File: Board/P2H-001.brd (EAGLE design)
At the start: 94.9 x 72.4 mm, 29 parts, among them IC1 74LS157N, IC2 LTC485N, IC3 74LS07N, IC4 LTC485N, IC5 4066N, IC6 TLC5941NT, IC7 TLC5941NT

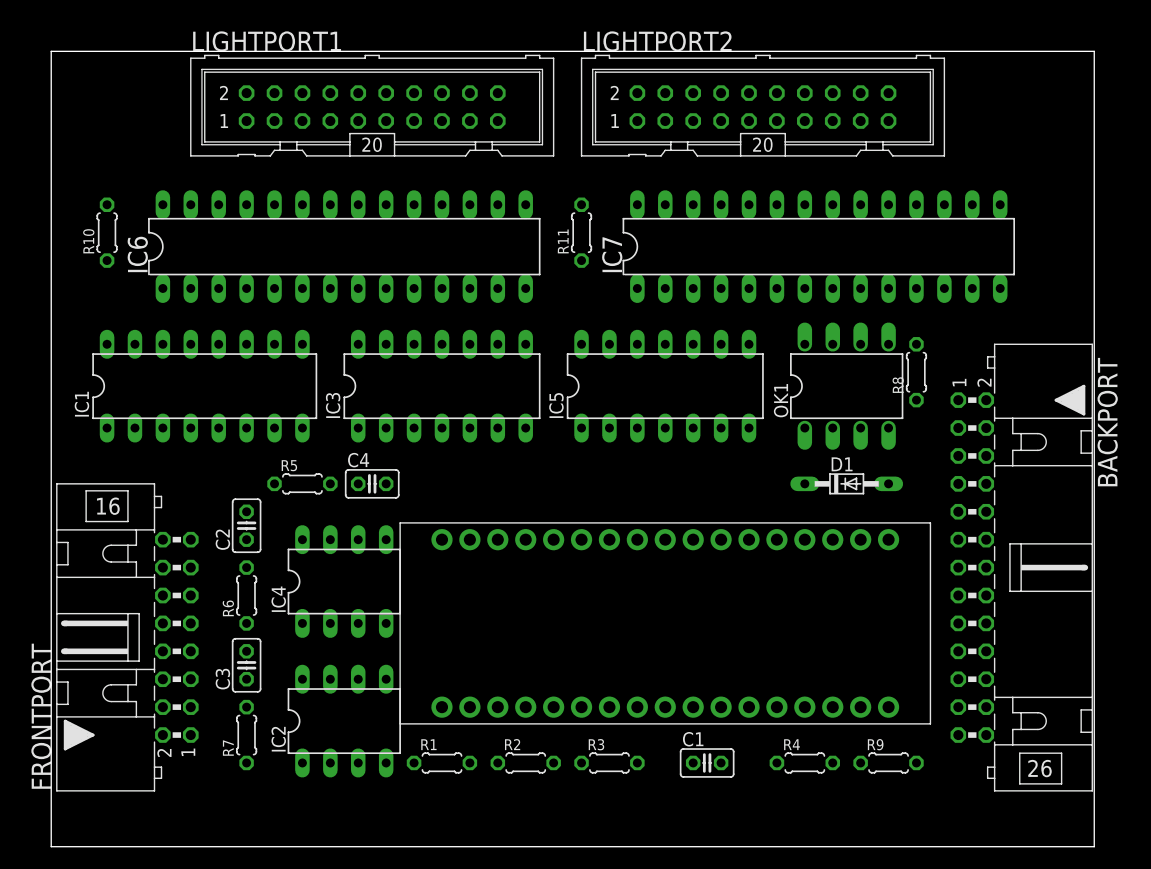
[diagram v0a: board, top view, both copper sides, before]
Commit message: Design renewed.
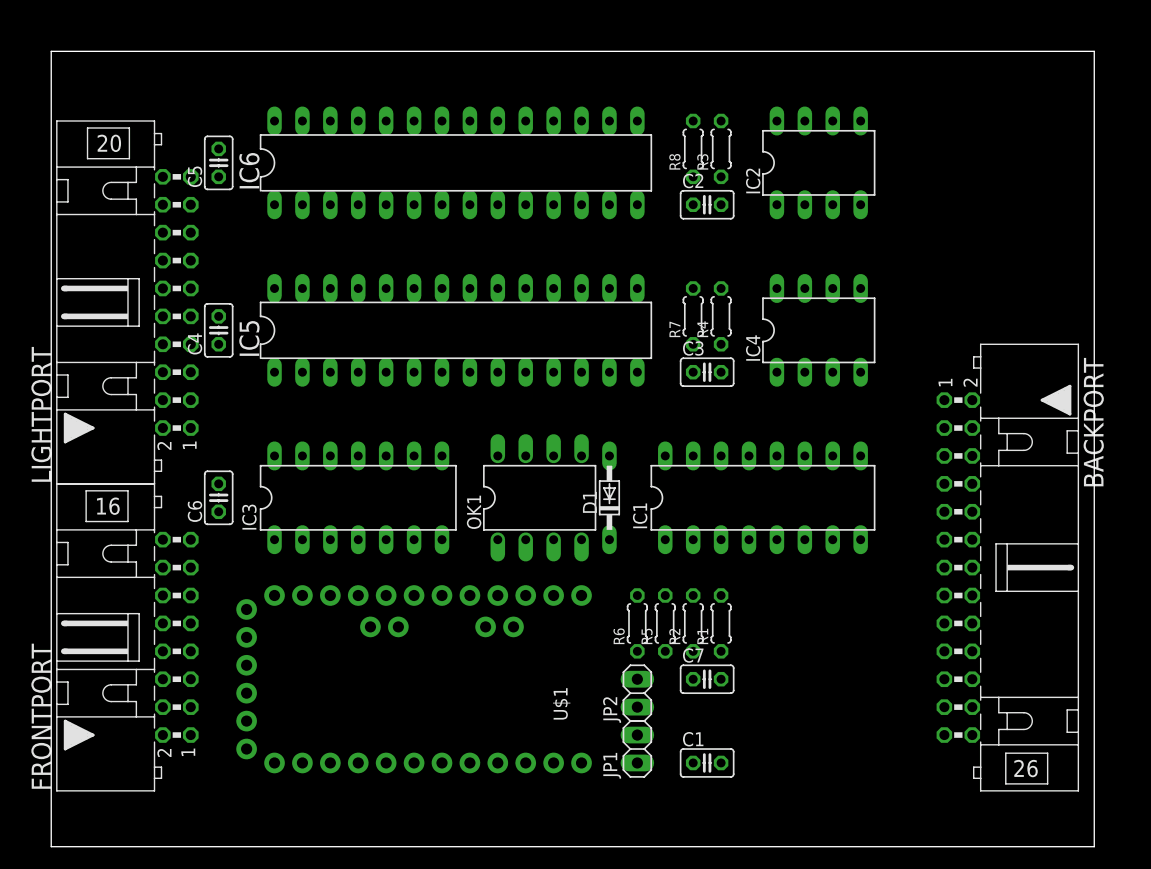
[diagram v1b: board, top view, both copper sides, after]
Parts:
- removed IC7: TLC5941NT, adafruit:DIL28-3
- removed LIGHTPORT1, LIGHTPORT2: (no value), con-ml:ML20
- removed MC1: ARDUINOMICRO, adafruit:ARDUINOMICRO
- removed R10, R11: 4.7k, resistor:0204/5
- removed R9: 220, resistor:0204/5
- added C5, C6, C7: (no value), rcl:C025-025X050
- added JP1, JP2: (no value), pinhead:1X02
- added LIGHTPORT: (no value), con-ml:ML20L
- added U$1: ARDUINO_PRO_MINI, SparkFun-Boards:ARDUINO_PRO_MINI
- IC5: value 4066N -> TLC5941NT; device 40xx:DIL14 -> adafruit:DIL28-3
- R1, R2: value 330 -> 220
- R3: value 330 -> 120
- R4: value 220 -> 120
- R5: value 10k -> 220
- R6: value 120 -> 220
- R7: value 120 -> 4.7k
- R8: value 220 -> 4.7k
- moved IC2 66.7 mm to (69.8, 62.2)
- moved R3 56.8 mm to (61.0, 63.5), turned to 90 degrees
- moved R7 55.7 mm to (58.4, 48.3)
- moved IC1 51.8 mm to (64.8, 31.8)
- moved C2 51.1 mm to (59.7, 58.4), turned to 0 degrees
- moved C3 49.7 mm to (59.7, 43.2), turned to 0 degrees
- moved IC4 48.9 mm to (69.8, 47.0)
- moved R4 41.3 mm to (61.0, 48.3), turned to 90 degrees
- moved R6 35.7 mm to (53.3, 20.3)
- moved R5 35.4 mm to (55.9, 20.3), turned to 90 degrees
- moved OK1 29.7 mm to (44.5, 31.8)
- moved R8 28.7 mm to (58.4, 63.5)
- moved R1 28.4 mm to (61.0, 20.3), turned to 90 degrees
- moved D1 21.6 mm to (50.8, 31.8), turned to 90 degrees
- moved R2 19.8 mm to (58.4, 20.3), turned to 90 degrees
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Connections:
- removed net 3V3: FRONTPORT.3, MC1.P$33
- removed net GPDETECT: BACKPORT.8, MC1.P$7
- removed net LEDMAX: FRONTPORT.13, R1.1
- removed net LEDMIN: FRONTPORT.11, R3.1
- removed net N$44: IC7.5, LIGHTPORT2.10
- removed net N$45: IC7.7, LIGHTPORT2.12
- removed net N$46: IC7.9, LIGHTPORT2.14
- removed net N$47: IC7.11, LIGHTPORT2.16
- removed net N$48: IC7.13, LIGHTPORT2.18
- removed net N$49: IC7.15, LIGHTPORT2.20
- removed net N$50: IC7.2, LIGHTPORT2.7
- removed net N$51: IC7.4, LIGHTPORT2.9
- removed net N$52: IC7.6, LIGHTPORT2.11
- removed net N$53: IC7.8, LIGHTPORT2.13
- removed net N$54: IC7.10, LIGHTPORT2.15
- removed net N$55: IC7.12, LIGHTPORT2.17
- removed net N$56: IC7.14, LIGHTPORT2.19
- removed net N$57: IC6.28, LIGHTPORT1.5
- removed net N$65: IC6.15, LIGHTPORT1.20
- removed net N$66: IC6.2, LIGHTPORT1.7
- removed net N$67: IC6.4, LIGHTPORT1.9
- removed net N$68: IC6.6, LIGHTPORT1.11
- removed net N$69: IC6.8, LIGHTPORT1.13
- removed net N$70: IC6.10, LIGHTPORT1.15
- removed net N$71: IC6.12, LIGHTPORT1.17
- removed net N$72: IC6.14, LIGHTPORT1.19
- removed net N$73: IC6.11, LIGHTPORT1.16
- removed net N$74: IC6.7, LIGHTPORT1.12
- removed net N$75: IC6.9, LIGHTPORT1.14
- removed net N$76: IC6.5, LIGHTPORT1.10
- removed net N$77: IC6.3, LIGHTPORT1.8
- removed net N$78: IC6.1, LIGHTPORT1.6
- removed net N$80: IC6.13, LIGHTPORT1.18
- removed net SCL: BACKPORT.15, MC1.P$10
- removed net SDA: BACKPORT.14, MC1.P$11
- removed net VR: FRONTPORT.16, MC1.P$9
- removed net VSS: IC5.7
- removed net XDETECT: BACKPORT.10, IC1.1, MC1.P$1, R5.1
- new net LED1B: FRONTPORT.10, IC5.2
- new net LED1G: FRONTPORT.9, IC5.1
- new net LED1R: FRONTPORT.8, IC5.28
- new net LED2B: FRONTPORT.13, IC5.5
- new net LED2G: FRONTPORT.12, IC5.4
- new net LED2R: FRONTPORT.11, IC5.3
- new net LED3B: FRONTPORT.16, IC5.8
- new net LED3G: FRONTPORT.15, IC5.7
- new net LED3R: FRONTPORT.14, IC5.6
- new net N$17: BACKPORT.18, U$1.13
- new net N$20: BACKPORT.26, D1.A, OK1.3
- new net N$22: BACKPORT.17, IC5.13
- new net N$23: FRONTPORT.7, U$1.A4
- new net N$24: IC5.14, LIGHTPORT.3
- new net N$25: IC5.15, LIGHTPORT.4
- new net N$26: IC6.28, LIGHTPORT.5
- new net N$27: IC6.2, LIGHTPORT.7
- new net N$28: IC6.4, LIGHTPORT.9
- new net N$29: IC6.6, LIGHTPORT.11
- new net N$30: IC6.8, LIGHTPORT.13
- new net N$31: IC6.10, LIGHTPORT.15
- new net N$32: IC6.12, LIGHTPORT.17
- new net N$33: IC6.14, LIGHTPORT.19
- new net N$34: IC6.1, LIGHTPORT.6
- new net N$35: IC6.3, LIGHTPORT.8
- new net N$36: IC6.5, LIGHTPORT.10
- new net N$40: IC6.9, LIGHTPORT.14
- new net SWRST: FRONTPORT.4, U$1.3
- new net XBAR: BACKPORT.5, IC1.1, U$1.11
- net BLANK: now also BACKPORT.4, IC5.23, U$1.7; no longer IC5.2, IC7.23
- net GND: now also C5.2, C6.2, C7.2, IC1.10, IC1.11, IC1.13, IC1.14, IC1.5, IC1.6, IC3.11, IC3.13, IC3.3, IC3.5, IC3.9, IC5.22, LIGHTPORT.2, U$1.23; no longer BACKPORT.4, FRONTPORT.10, FRONTPORT.12, FRONTPORT.14, FRONTPORT.4, FRONTPORT.6, FRONTPORT.8, IC7.22, LIGHTPORT1.2, LIGHTPORT1.4, LIGHTPORT2.2, LIGHTPORT2.4, MC1.P$12, MC1.P$21
- net GSCLCK: now also IC5.18, U$1.8; no longer BACKPORT.12, IC7.18, MC1.P$8
- net HSRX: now also IC1.3; no longer IC1.2
- net MIDIRX: now also IC1.2, JP2.2; no longer IC1.3
- net MODE: now also IC5.27, U$1.9; no longer IC5.9, IC7.27
- net N$1: now also IC1.4, JP1.2, JP2.1; no longer BACKPORT.3, MC1.P$31
- net N$10: now also BACKPORT.10, U$1.20; no longer FRONTPORT.5, MC1.P$22
- net N$11: now also BACKPORT.13, IC5.9; no longer BACKPORT.11, IC5.4, MC1.P$27
- net N$12: now also BACKPORT.14, IC5.10; no longer BACKPORT.13, IC5.8, MC1.P$26
- net N$13: now also R5.1; no longer R8.1
- net N$14: now also BACKPORT.15, IC5.11; no longer BACKPORT.19, R9.1
- net N$15: now also BACKPORT.24, R2.2; no longer BACKPORT.20, R4.2
- net N$16: now also IC5.17, IC6.26; no longer IC6.17, IC7.26
- net N$18: now also BACKPORT.25, R5.2; no longer BACKPORT.21, R8.2
- net N$19: now also BACKPORT.11, U$1.A6; no longer BACKPORT.17, MC1.P$19
- net N$2: now also R2.1; no longer R4.1
- net N$21: now also BACKPORT.16, IC5.12; no longer MC1.P$3, R1.2
- net N$3: now also BACKPORT.6, U$1.12; no longer FRONTPORT.15, R2.1
- net N$37: now also IC5.20, R7.2; no longer IC6.20, R10.2
- net N$38: now also IC6.20, R8.2; no longer IC7.20, R11.2
- net N$39: now also IC6.7, LIGHTPORT.12; no longer IC7.28, LIGHTPORT2.5
- net N$4: now also BACKPORT.23, R6.1; no longer BACKPORT.5, MC1.P$30
- net N$41: now also IC6.11, LIGHTPORT.16; no longer IC7.1, LIGHTPORT2.6
- net N$42: now also IC6.13, LIGHTPORT.18; no longer BACKPORT.22, D1.A, OK1.3
- net N$43: now also IC6.15, LIGHTPORT.20; no longer IC7.3, LIGHTPORT2.8
- net N$5: now also BACKPORT.12, U$1.A7; no longer MC1.P$4, R3.2
- net N$6: now also U$1.17; no longer MC1.P$29
- net N$7: now also FRONTPORT.3, R1.1; no longer MC1.P$34, R2.2
- net N$8: now also BACKPORT.8, U$1.18; no longer IC5.13, IC5.5, IC5.6, MC1.P$2
- net N$9: now also U$1.19; no longer IC5.1, MC1.P$28
- net RX: now also JP1.1, U$1.2; no longer IC1.4, MC1.P$14
- net RX+: now also BACKPORT.19, R4.1; no longer BACKPORT.23, R7.1
- net RX-: now also BACKPORT.20, R4.2; no longer BACKPORT.24, R7.2
- net SCLCK: now also IC5.25, U$1.16; no longer BACKPORT.18, IC7.25, MC1.P$18
- net SIN: now also IC5.26, U$1.14; no longer BACKPORT.16, IC6.26, MC1.P$17
- net SWMAX: now also FRONTPORT.6, U$1.6; no longer FRONTPORT.9, MC1.P$5
- net SWMIN: now also FRONTPORT.5, U$1.5; no longer FRONTPORT.7, MC1.P$6
- net TX: now also U$1.1; no longer MC1.P$15
- net TX+: now also BACKPORT.21, R3.1; no longer BACKPORT.25, R6.1
- net TX-: now also BACKPORT.22, R3.2; no longer BACKPORT.26, R6.2
- net VCC: now also BACKPORT.1, C5.1, C6.1, C7.1, IC5.19, IC5.21, R6.2, R7.1, R8.1, U$1.21; no longer BACKPORT.6, IC7.19, IC7.21, MC1.P$23, R10.1, R11.1, R5.2, R9.2
- net VDD: now also BACKPORT.3, LIGHTPORT.1, R1.2, U$1.24; no longer BACKPORT.1, IC5.14, LIGHTPORT1.1, LIGHTPORT1.3, LIGHTPORT2.1, LIGHTPORT2.3, MC1.P$20
- net XLAT: now also IC5.24, U$1.10; no longer IC5.3, IC7.24
